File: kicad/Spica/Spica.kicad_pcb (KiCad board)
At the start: 2 copper layers, 61 x 61 mm, 13 parts, among them IC1 TA48033S, M1 Motor_DC, M2 Motor_DC, SW1 SW_SPDT, U1 ESP32-DEVKITC-32D, U2 DRV8835-akizuki, U3 HC-SR04, U4 AE-XCL102D503CR-G

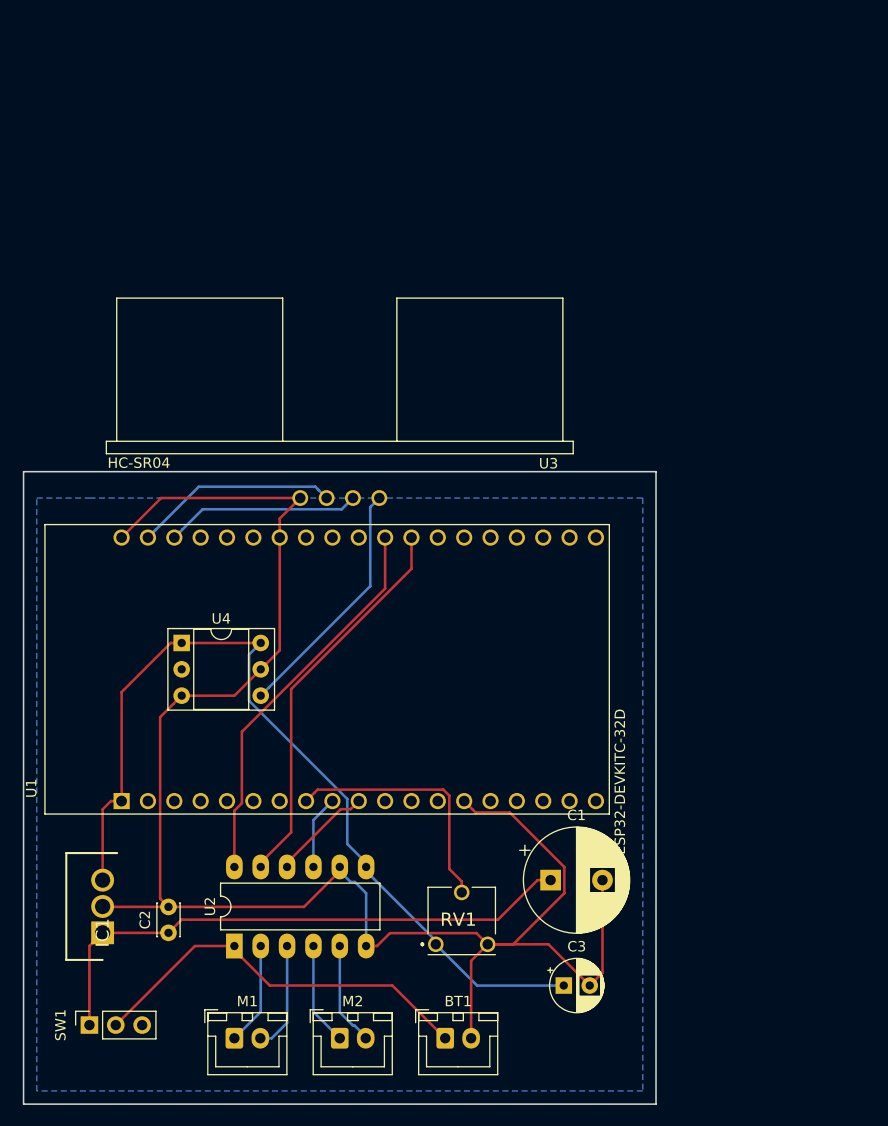
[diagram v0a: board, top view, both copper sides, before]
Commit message: ベタパターンを追加
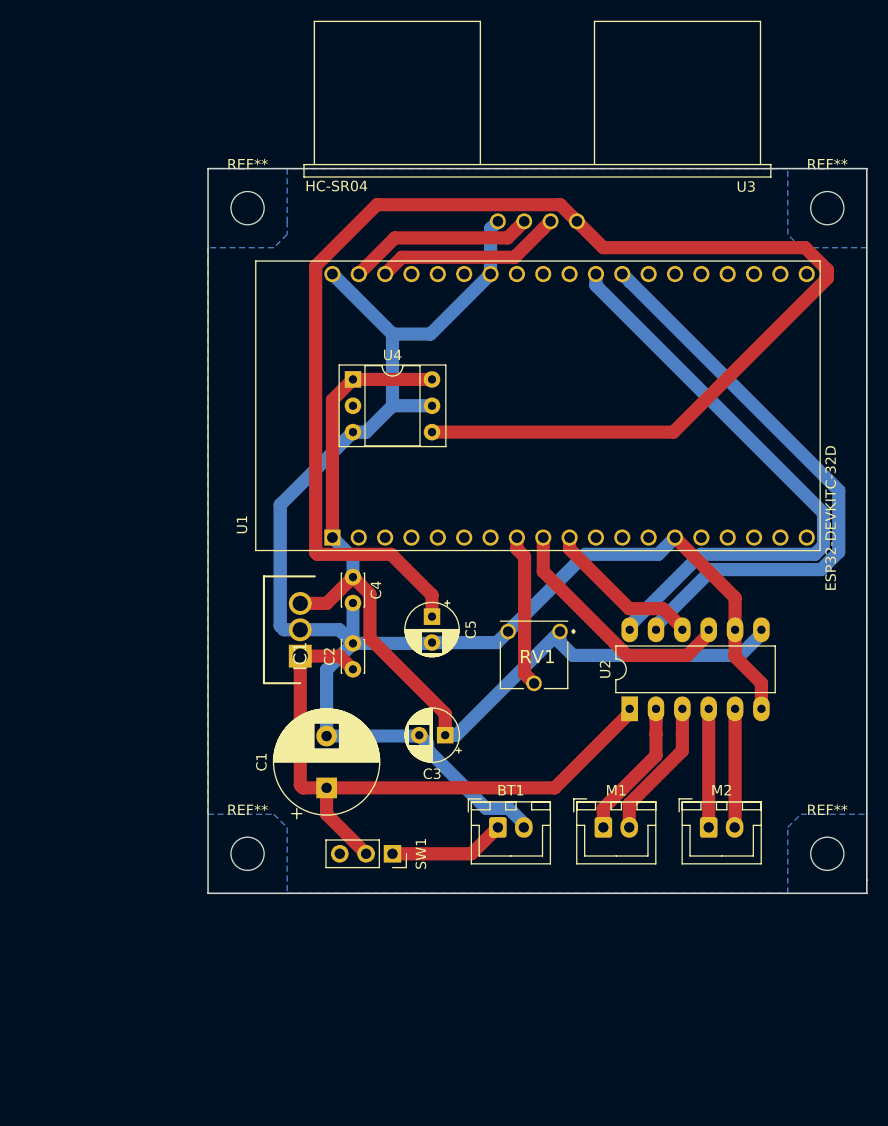
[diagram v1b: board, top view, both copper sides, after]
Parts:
- added C4: 0.1μ, Capacitor_THT:C_Disc_D3.0mm_W2.0mm_P2.50mm, F.Cu at (151.1, 99.1)
- added C5: 10μ, Capacitor_THT:CP_Radial_D5.0mm_P2.50mm, F.Cu at (158.8, 102.9)
- added REF**: MountingHole_3.2mm_M3, MountingHole:MountingHole_3.2mm_M3, F.Cu at (196.8, 63.5)
- added REF**: MountingHole_3.2mm_M3, MountingHole:MountingHole_3.2mm_M3, F.Cu at (196.8, 125.7)
- added REF**: MountingHole_3.2mm_M3, MountingHole:MountingHole_3.2mm_M3, F.Cu at (141.0, 125.7)
- added REF**: MountingHole_3.2mm_M3, MountingHole:MountingHole_3.2mm_M3, F.Cu at (141.0, 63.5)
- moved U2 44.4 mm to (177.8, 111.8)
- moved M1 41.0 mm to (175.3, 123.2)
- moved M2 41.0 mm to (185.4, 123.2)
- moved SW1 33.6 mm to (154.9, 125.7), turned to 270 degrees
- moved IC1 32.8 mm to (146.1, 106.7)
- moved U3 32.8 mm to (168.9, 64.8)
- moved U1 32.5 mm to (168.9, 82.5)
- moved C2 31.0 mm to (151.1, 108.0)
- moved U4 30.3 mm to (151.1, 80.0)
- moved C3 26.7 mm to (160.0, 114.3), turned to 180 degrees
- moved RV1 26.5 mm to (168.9, 106.7), turned to 180 degrees
- moved C1 23.3 mm to (148.6, 119.4), turned to 90 degrees
- moved BT1 20.9 mm to (165.1, 123.2)
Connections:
- BT1 pad 1: VCC -> Net-(BT1-Pad1)
- C1 pad 1: Net-(C1-Pad1) -> VCC
- C2 pad 1: Net-(C1-Pad1) -> VCC
- IC1 pad 1: Net-(C1-Pad1) -> VCC
- SW1 pad 1: Net-(C1-Pad1) -> Net-(BT1-Pad1)
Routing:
- net 5V: track 23.8 -> 142.0 mm
- net Net-(C1-Pad1): track 54.7 -> 0.00 mm
- net VCC: track 38.8 -> 61.2 mm
- net IO17: track 37.8 -> 57.5 mm
- net IO16: track 37.8 -> 56.4 mm
- net IO25: track 7.11 -> 23.8 mm
- net Net-(BT1-Pad1): track 0.00 -> 11.2 mm
- net Net-(RV1-Pad2): track 24.3 -> 14.7 mm
- net GND: track 169.5 -> 163.2 mm
- net IO26: track 9.77 -> 15.3 mm
- net 3.3V: track 85.8 -> 90.8 mm
- net Net-(M1-Pad1): track 9.94 -> 14.5 mm
- net Net-(M1-Pad2): track 10.6 -> 14.3 mm
- net IO23: track 20.8 -> 18.1 mm
- net Net-(M2-Pad2): track 10.0 -> 11.8 mm
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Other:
- board size 61 x 61 mm -> 63.5 x 69.8 mm
- net class Default: trace_width 0.25 -> 1.27

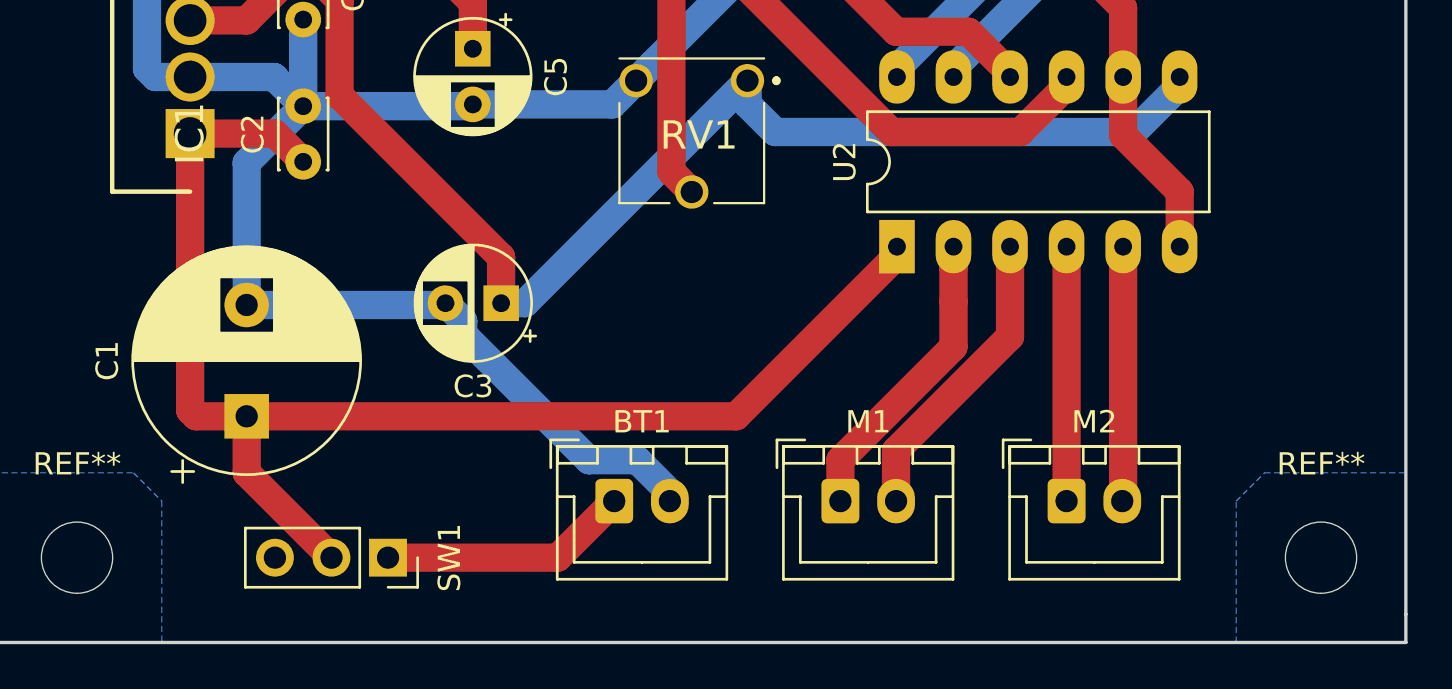
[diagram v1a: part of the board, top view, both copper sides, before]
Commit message: 細かな修正
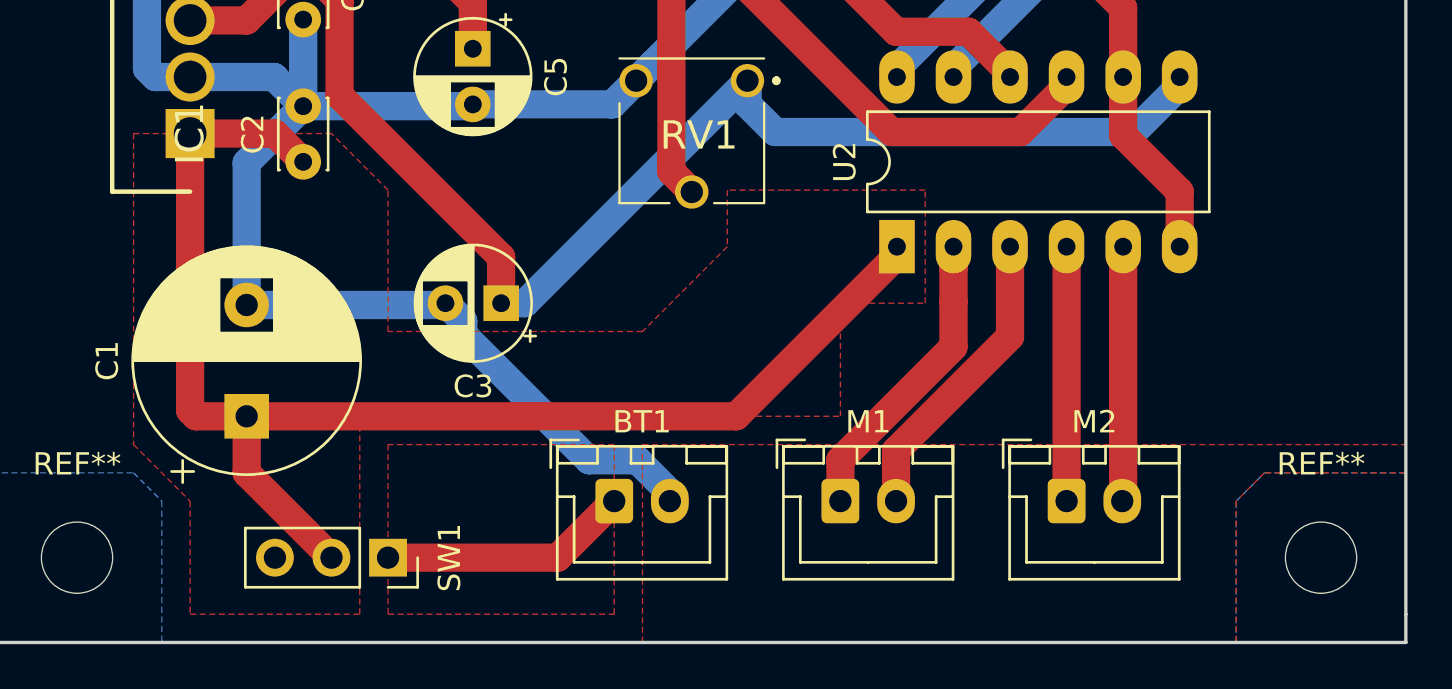
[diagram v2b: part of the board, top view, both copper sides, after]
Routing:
- added copper zone on F.Cu, net GND
- added copper zone on F.Cu, net Net-(BT1-Pad1)
- added copper zone on F.Cu, net VCC
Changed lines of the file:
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@@
+    )
+  )
+  (zone (net 45) (net_name "Net-(BT1-Pad1)") (layer F.Cu) (hatch edge 0.508)
+    (connect_pads yes (clearance 0.508))
+    (min_thickness 0.254)
+    (fill yes (arc_segments 16) (thermal_gap 0.508) (thermal_bridge_width 0.508) (smoothing fillet) (radius 1))
+    (polygon
+      (pts
+        (xy 154.94 120.65) (xy 154.94 128.27) (xy 165.1 128.27) (xy 165.1 120.65)
+      )
+    )
+  )
+  (zone (net 1) (net_name VCC) (layer F.Cu) (hatch edge 0.508)
+    (connect_pads yes (clearance 0.508))
+    (min_thickness 0.254)
+    (fill yes (arc_segments 16) (thermal_gap 0.508) (thermal_bridge_width 0.508) (smoothing fillet) (radius 1))
+    (polygon
+      (pts
+        (xy 153.67 128.27) (xy 153.67 119.38) (xy 170.18 119.38) (xy 175.26 119.38) (xy 175.26 114.3)
+        (xy 179.07 114.3) (xy 179.07 109.22) (xy 172.72 109.22) (xy 170.18 109.22) (xy 170.18 111.76)
+        (xy 166.37 115.57) (xy 154.94 115.57) (xy 154.94 109.22) (xy 152.4 106.68) (xy 143.51 106.68)
+        (xy 143.51 120.65) (xy 146.05 123.19) (xy 146.05 128.27)
+      )
+    )
+  )
+  (zone (net 2) (net_name GND) (layer F.Cu) (hatch edge 0.508)
+    (connect_pads (clearance 0.508))
+    (min_thickness 0.254)
+    (fill yes (arc_segments 16) (thermal_gap 0.508) (thermal_bridge_width 0.508))
+    (polygon
+      (pts
+        (xy 166.37 129.54) (xy 166.37 120.65) (xy 200.66 120.65) (xy 200.66 121.92) (xy 194.31 121.92)
+        (xy 193.04 123.19) (xy 193.04 129.54)
+      )
     )
   )
